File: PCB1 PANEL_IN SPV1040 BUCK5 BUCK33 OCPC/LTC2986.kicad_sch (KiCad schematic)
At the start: 1 part, among them U15 LTC2986HLX_PBF

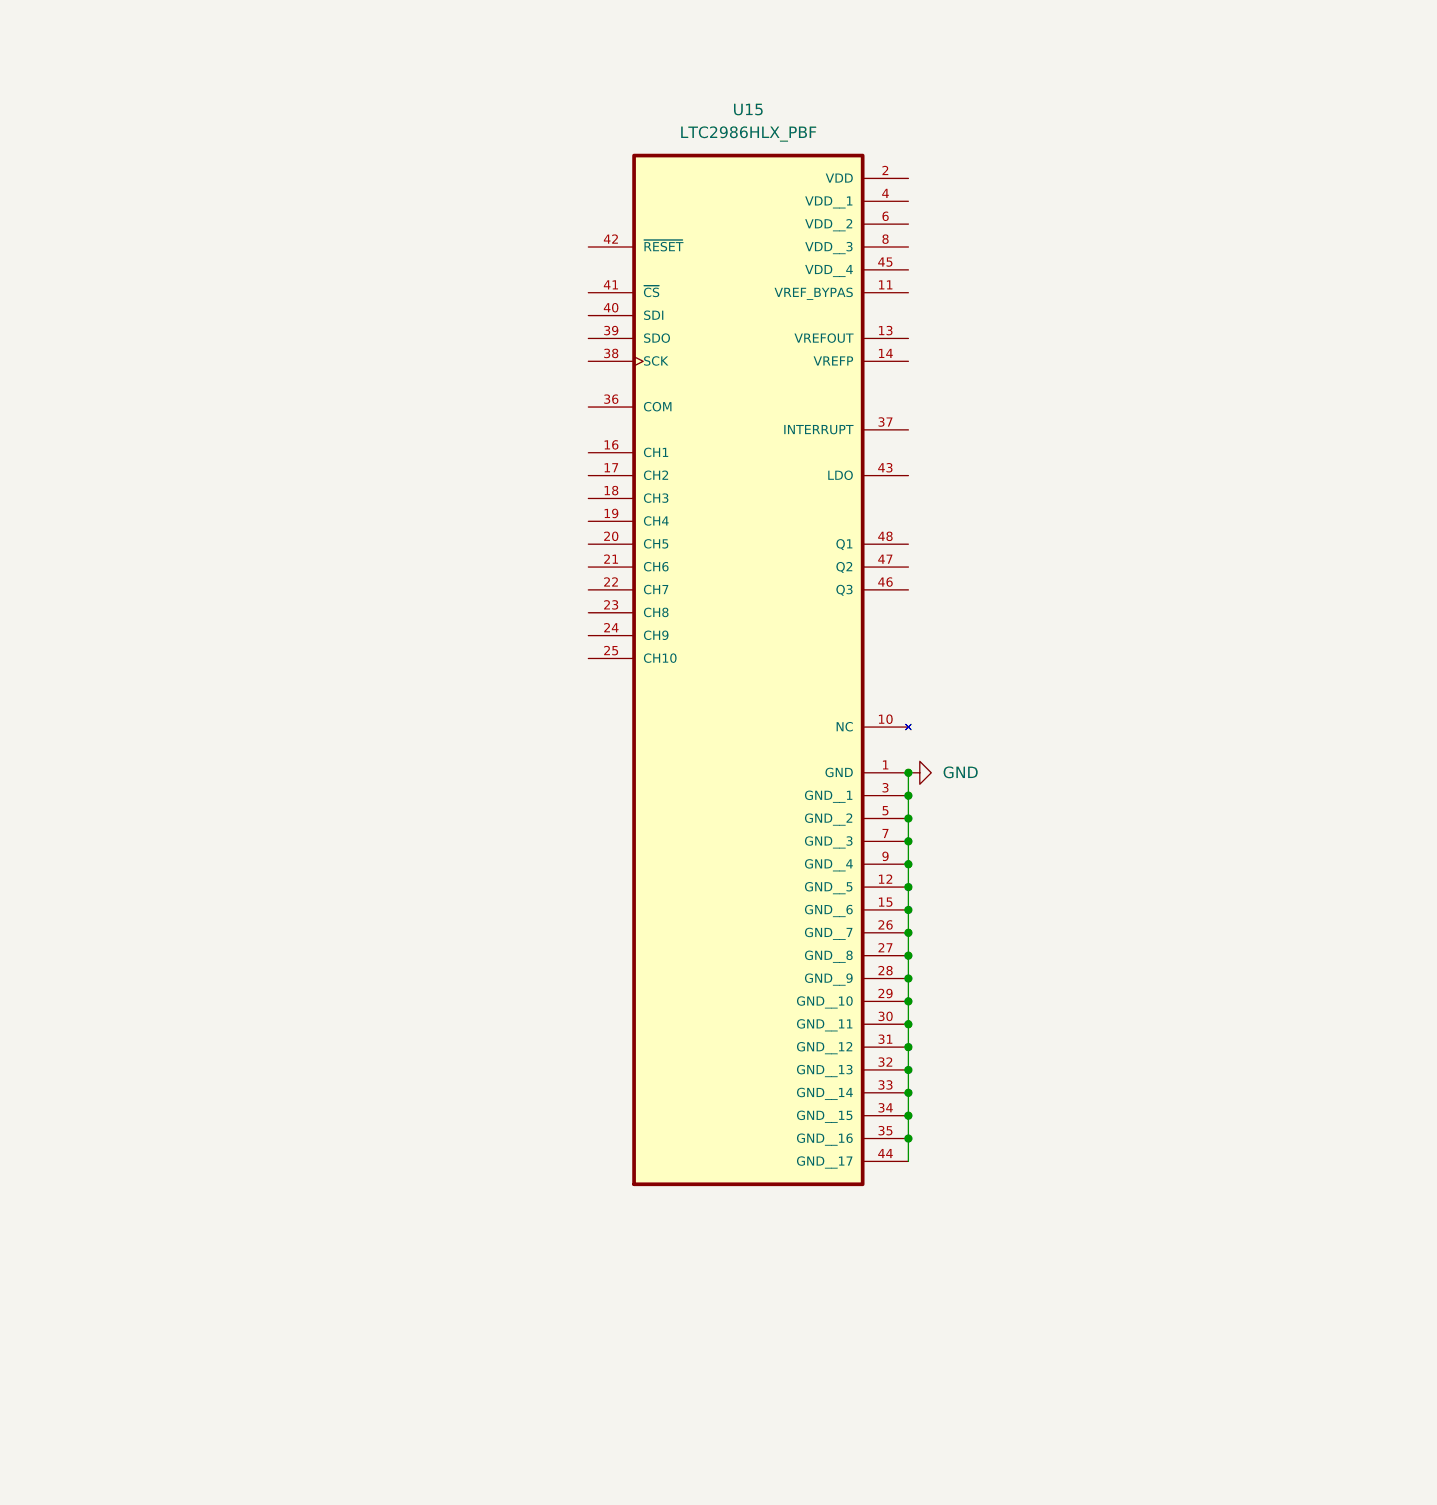
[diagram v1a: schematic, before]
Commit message: s
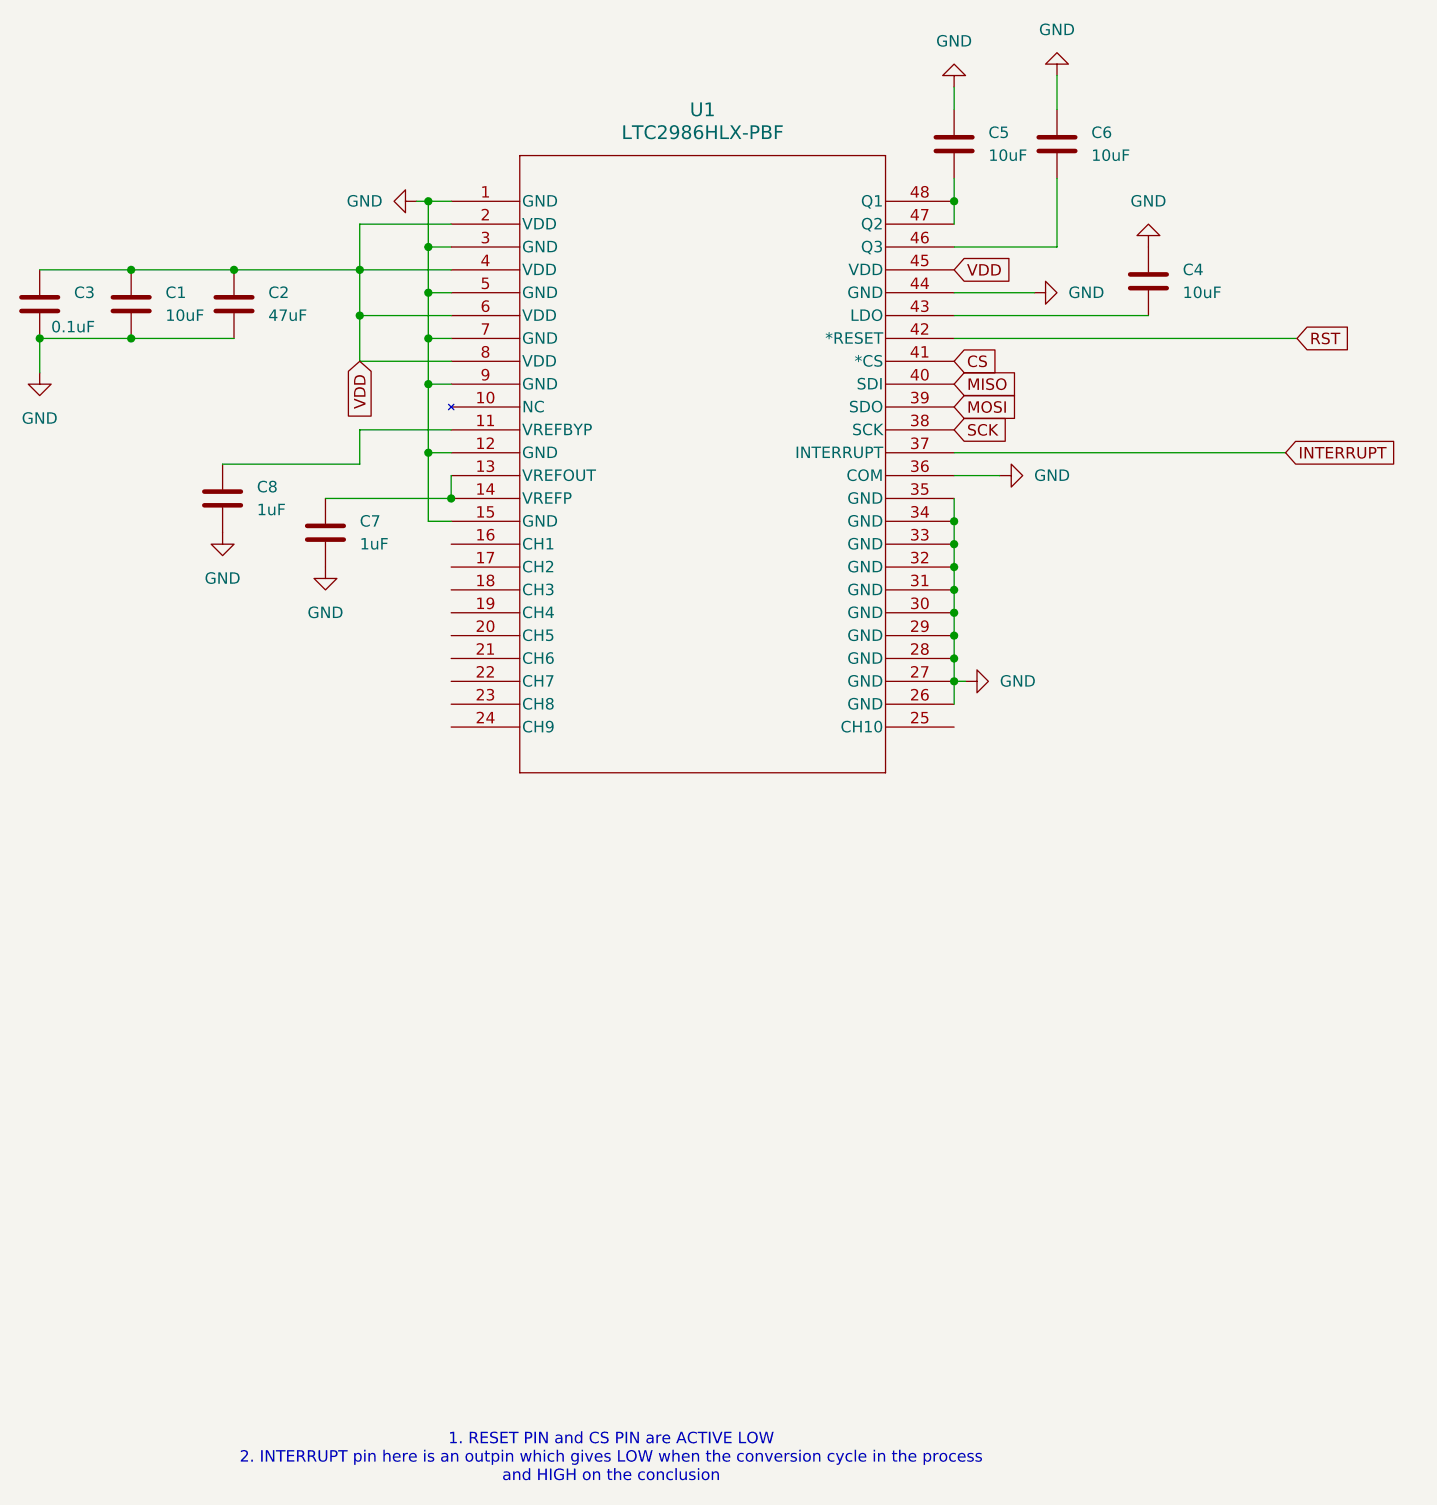
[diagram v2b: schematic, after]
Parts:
- removed U15: LTC2986HLX_PBF, LTC2986HLX_PBF:QFP50P900X900X160-48N, symbol LTC2986:LTC2986HLX_PBF
- added C1, C4, C5, C6: 10uF, symbol Device:C
- added C2: 47uF, symbol Device:C
- added C3: 0.1uF, symbol Device:C
- added C7, C8: 1uF, symbol Device:C
- added U1: LTC2986HLX-PBF, LX_48_ADI, symbol 2025-01-09_17-24-37:LTC2986HLX-PBF
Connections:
- net GND: now also C1.2, C2.2, C3.2, C4.2, C5.2, C6.2, C7.2, C8.2, U1.1 (GND), U1.12 (GND), U1.15 (GND), U1.26 (GND), U1.27 (GND), U1.28 (GND), U1.29 (GND), U1.3 (GND), U1.30 (GND), U1.31 (GND), U1.32 (GND), U1.33 (GND), U1.34 (GND), U1.35 (GND), U1.36 (COM), U1.44 (GND), U1.5 (GND), U1.7 (GND), U1.9 (GND)
- new net: C8.1, U1.11 (VREFBYP)
- new net: C7.1, U1.13 (VREFOUT), U1.14 (VREFP)
- new net: C4.1, U1.43 (LDO)
- new net: C6.1, U1.46 (Q3)
- new net: C5.1, U1.47 (Q2), U1.48 (Q1)
- new net CS: U1.41 (*CS)
- new net INTERRUPT: U1.37 (INTERRUPT)
- new net MISO: U1.40 (SDI)
- new net MOSI: U1.39 (SDO)
- new net RST: U1.42 (*RESET)
- new net SCK: U1.38 (SCK)
- new net VDD: C1.1, C2.1, C3.1, U1.2 (VDD), U1.4 (VDD), U1.45 (VDD), U1.6 (VDD), U1.8 (VDD)
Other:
- note added: "1. RESET PIN and CS PIN are ACTIVE LOW 2. INTERRUPT pin here is an outpin which gives LOW when the conversion cycle in the process and HIGH on the conclusion"
